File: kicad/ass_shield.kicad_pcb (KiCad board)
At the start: 2 copper layers, 100 x 86 mm, 210 parts, among them J1 Conn_01x03_Male, J10 HEADER_1x4, J11 HEADER-1x08, J12 U.FL, J13 RJ11-6PTH, J14 U.FL, J15 HEADER-1x02, J16 Conn_01x03_Male, J17 Conn_01x40_Male, J18 Conn_01x38_Male, J19 HEADER-1x02-connectors, J2 DEBUG, J20 HEADER_1x4, J3 Conn_01x03_Male, J4 USB, J5 U.FL, J6 USB, J7 USBMINI, J8 U.FL, J9 RJ45, M1 CR1220SMD, P1 HEADER_2x5, Q1 BSN20, Q2 BC107, SW1 SW_DIP-8-SMT-HALFSIZE, SW2 SW_DIP-8-SMT-HALFSIZE, U1 OrangePiPC, U10 MCP2515-EST, U11 MCP2551-I-SN, U12 MCP3424, U13 MCP3424, U14 MCP3424, U15 MCP3424, U16 MCP23017-E_SO, U17 LM2596S-5, U18 LM1117-3.3, U19 CP2102-GMR_NRND, U2 DS3231M, U20 PCA9685, U21 MCP4728, U22 MCP4728, U23 MCP4728, U24 MCP4728, U3 SN65HVD72, U4 NRF24L01p, U5 RFM95HW, U6 CC2530F, U7 DS2482, U8 DS9503, U9 RFM69HW, Y1 9,84375 MHz, Y2 13,5600 MHz, Y3 4,8970 MHz, Y4 6,7458 MHz, Y5 32 MHz, Y6 16 MHz, Y7 16 MHz

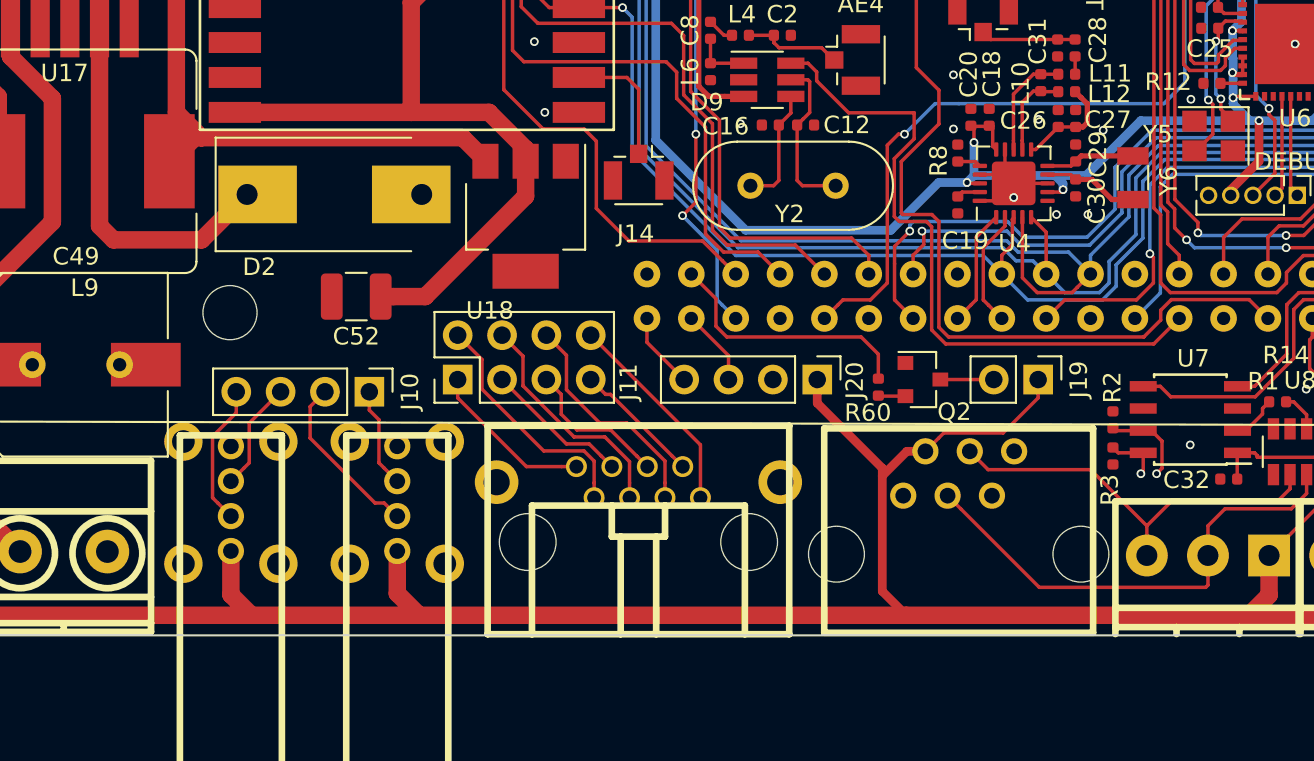
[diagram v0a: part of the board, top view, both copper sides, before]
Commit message: a msg
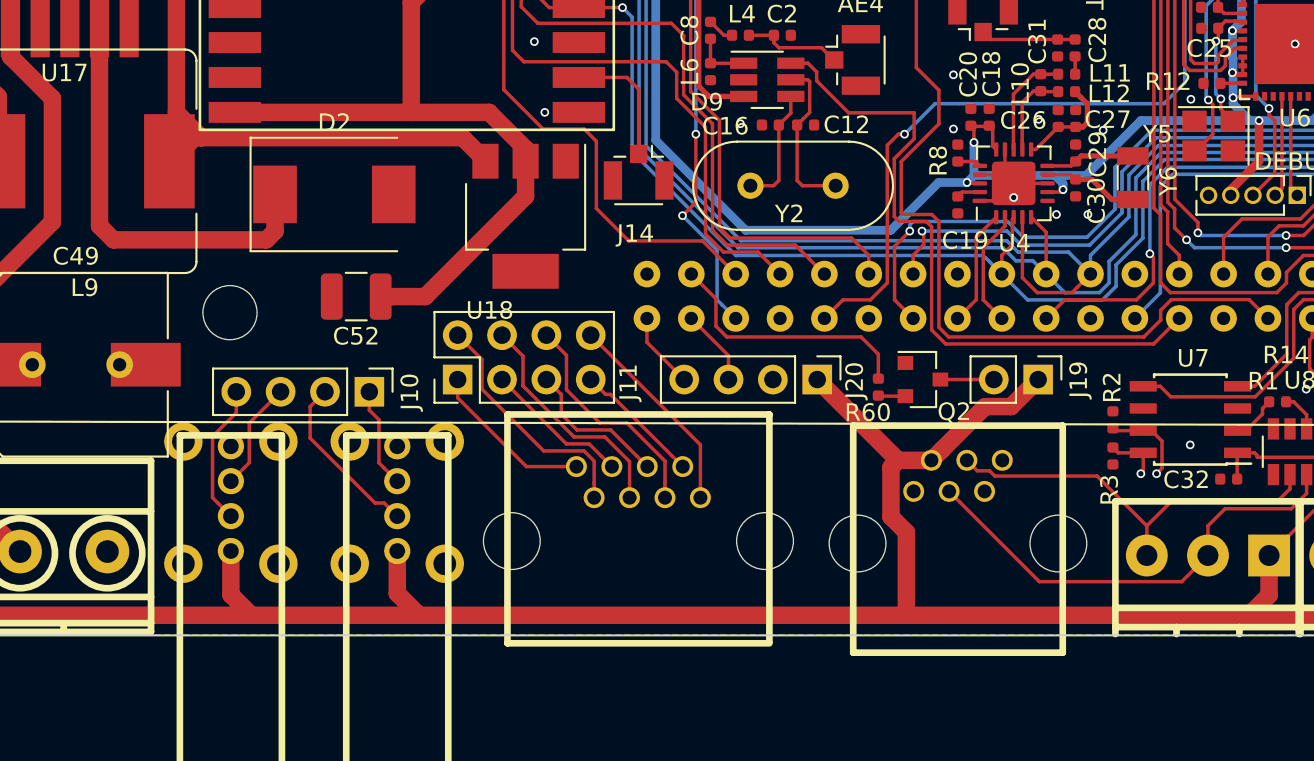
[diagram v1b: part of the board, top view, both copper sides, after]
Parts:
- C10, C9: value 0,047 µF -> 47 nF
- C17, C21: value 22pF -> 22 pF
- C22, C33: value 560pF -> 560 pF
- C32, C53, C57, C58, C59, C60, C61, C64: value 100nF -> 100 nF
- C34, C40, C42, C44, C62, C63: value 100uF -> 100 nF
- C35, C41, C43, C46: value 10uF -> 10 uF
- C49: value 680 uF -> 680 µF
- C51, C52: value 220 uF -> 220 µF
- D2: footprint Diode_SMD:D_SMC-RM10_Universal_Handsoldering -> Diode_SMD:D_SMC
- J13: footprint imm:6p6c -> imm:rj11-shield
- J9: footprint w_conn_pc:rj45-shield -> imm:rj45-shield
- R1: value 100 -> 100 R
- R10, R11: value 100R -> 100 R
- R14, R19, R2, R21, R23, R25, R27, R29, R3, R31, R33, R35, R36, R37, R38, R39, R40, R41, R43, R45, R47, R49, R5, R51, R53, R55, R57, R58, R59, R7: value 10k -> 10 k
- R15, R16: value 10R -> 10 R
- R17, R18: value 120R -> 120 R
- R20, R22, R24, R26, R28, R30, R32, R34, R42, R44, R46, R48, R50, R52, R54, R56: value 6.8k -> 6,8 k
- R4: value 0 -> 0 R
- R6: value 22k -> 22 k
- R9: value 4.7k -> 4,7 k
- moved J13 1.11 mm to (153.3, 131.2)
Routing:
- net Net-(D2-Pad1): track 45.6 -> 48.5 mm
- net 5V: track 691.7 -> 690.1 mm
- net Net-(J13-Pad3): track 28.0 -> 26.8 mm
